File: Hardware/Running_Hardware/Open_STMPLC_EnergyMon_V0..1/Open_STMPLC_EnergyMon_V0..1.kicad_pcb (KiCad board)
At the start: 2 copper layers, 63 x 82 mm, 122 parts, among them J1 Conn_02x08_Odd_Even, J2 Screw_Terminal_01x08, U1 ATM90E36A, U2 ISO7762FDBQ, U5 AMS1117-3.3, Y1 16.384MHz

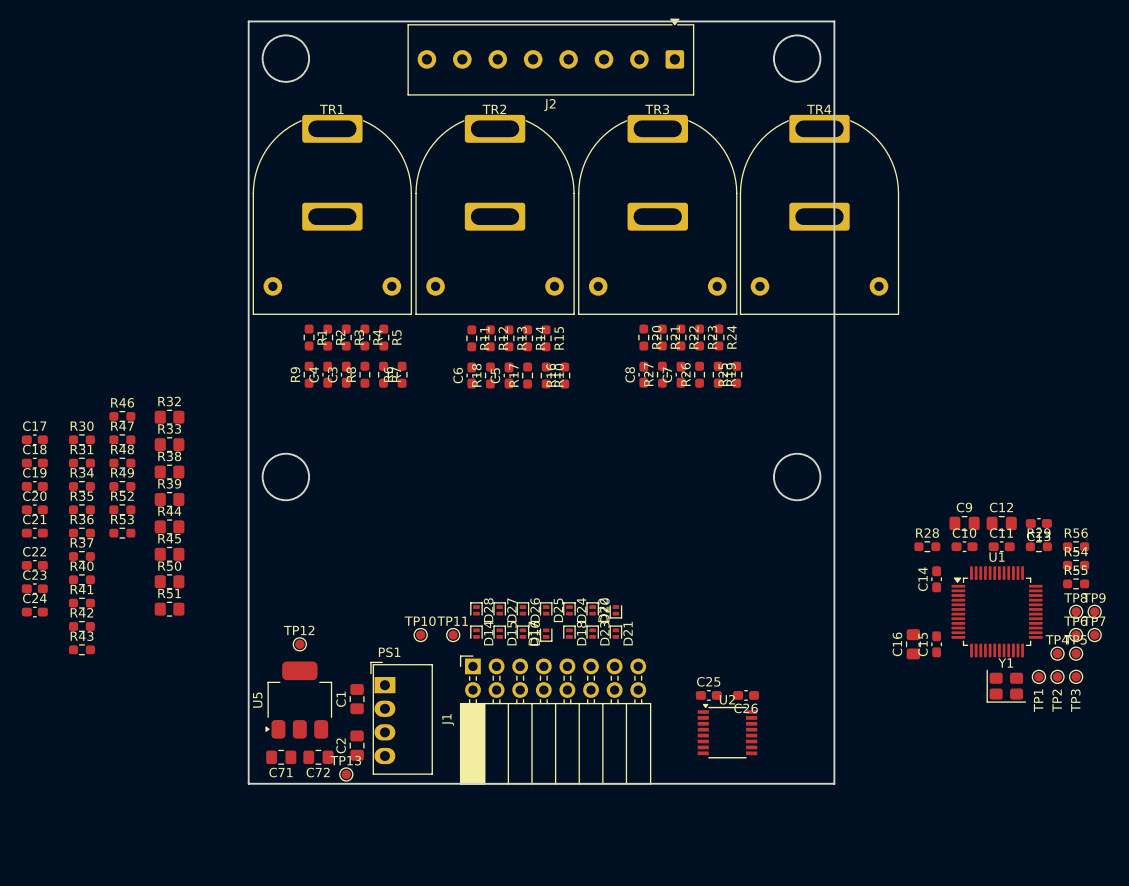
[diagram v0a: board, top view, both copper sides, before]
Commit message: Energy monitoring layout
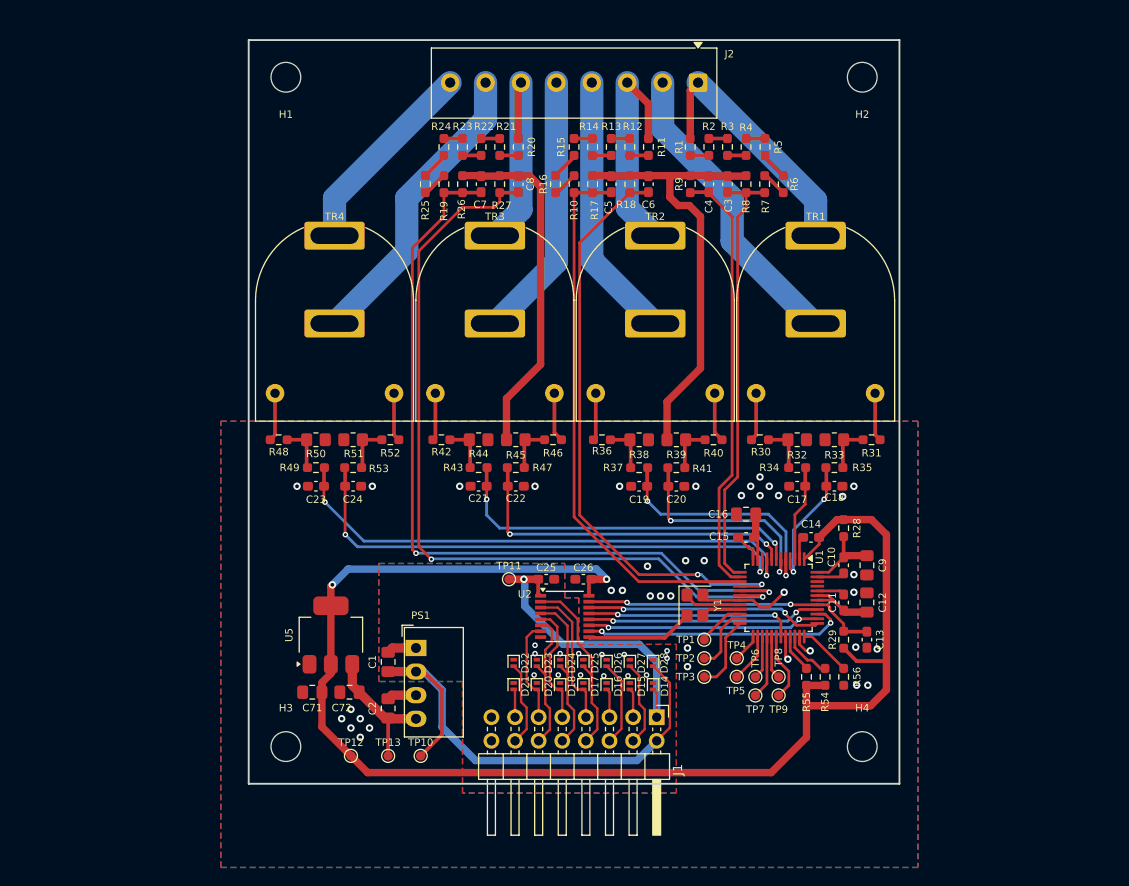
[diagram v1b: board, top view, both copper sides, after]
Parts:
- added H1: MountingHole, MountingHole:MountingHole_3.2mm_M3, F.Cu at (94.0, 64.0)
- added H2: MountingHole, MountingHole:MountingHole_3.2mm_M3, F.Cu at (156.0, 64.0)
- added H3: MountingHole, MountingHole:MountingHole_3.2mm_M3, F.Cu at (94.0, 136.0)
- added H4: MountingHole, MountingHole:MountingHole_3.2mm_M3, F.Cu at (156.0, 136.0)
- J1: footprint Connector_PinSocket_2.54mm:PinSocket_2x08_P2.54mm_Horizontal -> Connector_PinHeader_2.54mm:PinHeader_2x08_P2.54mm_Horizontal
- moved C18 86.0 mm to (153.0, 108.0)
- moved R31 85.0 mm to (157.0, 103.0), turned to 180 degrees
- moved C17 82.2 mm to (149.0, 108.0), turned to 180 degrees
- moved R35 81.1 mm to (153.0, 106.0)
- moved R34 77.0 mm to (149.0, 106.0), turned to 180 degrees
- moved R30 72.9 mm to (145.0, 103.0)
- moved R33 71.5 mm to (153.0, 103.0), turned to 180 degrees
- moved R40 69.6 mm to (140.0, 103.0), turned to 180 degrees
- moved C20 69.0 mm to (136.0, 108.0)
- moved R32 67.6 mm to (149.0, 103.0), turned to 180 degrees
- moved R41 65.6 mm to (136.0, 106.0)
- moved C19 65.0 mm to (132.0, 108.0), turned to 180 degrees
- moved R37 60.7 mm to (132.0, 106.0), turned to 180 degrees
- moved R36 56.8 mm to (128.0, 103.0)
- moved R39 54.9 mm to (136.0, 103.0), turned to 180 degrees
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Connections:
- C26 pad 2: GND -> GNDA
- J2 pad 1: /N_OUT -> /U_IN
- J2 pad 2: /N_IN -> /U_OUT
- J2 pad 3: /W_OUT -> /V_IN
- J2 pad 4: /W_IN -> /V_OUT
- J2 pad 5: /V_OUT -> /W_OUT
- J2 pad 6: /V_IN -> /W_IN
- J2 pad 7: /U_OUT -> /N_OUT
- J2 pad 8: /U_IN -> /N_IN
- U2 pad 10: /IRQ0 -> /SDO
- U2 pad 11: /SDO -> /SCLK
- U2 pad 12: /SCLK -> /SDI
- U2 pad 13: /SDI -> /IRQ0
- U2 pad 2: /EX_GPIO1 -> /EX_GPIO3
- U2 pad 4: /EX_SPI_MOSI -> /EX_GPIO1
- U2 pad 5: /EX_SPI_CLK -> /EX_SPI_MOSI
- U2 pad 6: /EX_SPI_MISO -> /EX_SPI_CLK
- U2 pad 7: /EX_GPIO3 -> /EX_SPI_MISO
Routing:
- net +3.3VA: track 0.00 -> 156.1 mm, vias 0 -> 2
- net GNDA: track 0.00 -> 127.5 mm, vias 0 -> 39
- net /VCN: track 0.00 -> 87.5 mm, vias 0 -> 2
- net /VCP: track 0.00 -> 87.3 mm, vias 0 -> 2
- net /VBN: track 0.00 -> 64.1 mm, vias 0 -> 2
- net /VBP: track 0.00 -> 59.6 mm
- net /INP: track 0.00 -> 57.6 mm, vias 0 -> 2
- net +5V: track 0.00 -> 57.1 mm
- net /INN: track 0.00 -> 55.8 mm, vias 0 -> 2
- net /VAP: track 0.00 -> 46.9 mm
- net /VAN: track 0.00 -> 46.5 mm
- net /ICP: track 0.00 -> 39.2 mm, vias 0 -> 2
- net /ICN: track 0.00 -> 37.2 mm, vias 0 -> 2
- net +3V3: track 0.00 -> 33.7 mm, vias 0 -> 1
- net /U_OUT: track 0.00 -> 32.8 mm
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- added copper zone on B.Cu, net GND
- added copper zone on F.Cu, net GND
- added copper zone on B.Cu, net GNDA
- added copper zone on F.Cu, net GNDA
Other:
- board size 63 x 82 mm -> 70 x 80 mm
